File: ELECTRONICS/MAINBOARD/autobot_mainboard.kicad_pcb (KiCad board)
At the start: 4 copper layers, 62 x 42.5 mm, 161 parts, among them IC1 DW3210, J1 USB_C_Receptacle_USB2.0_16P, J10 Conn_01x05_Socket, J12 Conn_01x02_Pin, J14 Conn_01x05_Pin, J16 Conn_01x05_Pin, J17 Conn_01x02_Pin, J18 Conn_01x02_Pin, J19 Conn_02x05_Odd_Even, J20 Conn_02x05_Odd_Even, J7 Conn_01x03_Pin, J8 Conn_Coaxial, J9 Conn_Coaxial, Q1 DMG1012T, Q2 DMG1012T, Q3 DMG1012T, SW1 RESET, SW2 BOOT, U1 TVS1400DRV, U10 VL53L1X, U11 VL53L1X, U12 VL53L1X, U13 BMI270, U14 BMI270, U15 TPD4E05U06DQA, U16 LP5907MFX-3.3, U17 STM32G031C6Tx, U18 LP5907MFX-3.3, U19 STM32H743VITx, U2 LMR51430XDDCR, U22 TPD4E05U06DQA, U23 LP5907MFX-3.3, U3 LP5907MFX-3.3, U4 TPD2EUSB30A, U9 VL53L1X, Y1 TXC 8Y38472012, Y2 25mhz placeholder

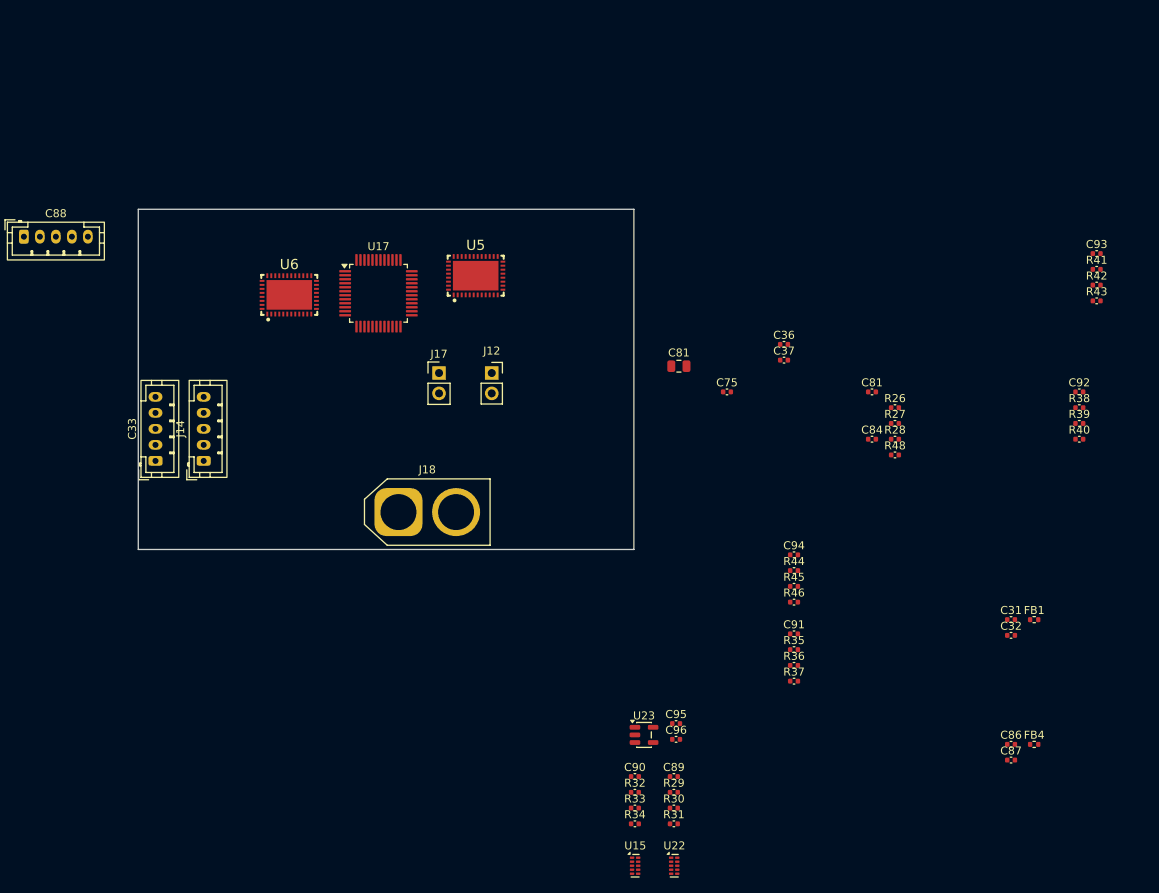
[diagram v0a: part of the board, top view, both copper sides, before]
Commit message: driver board schematic
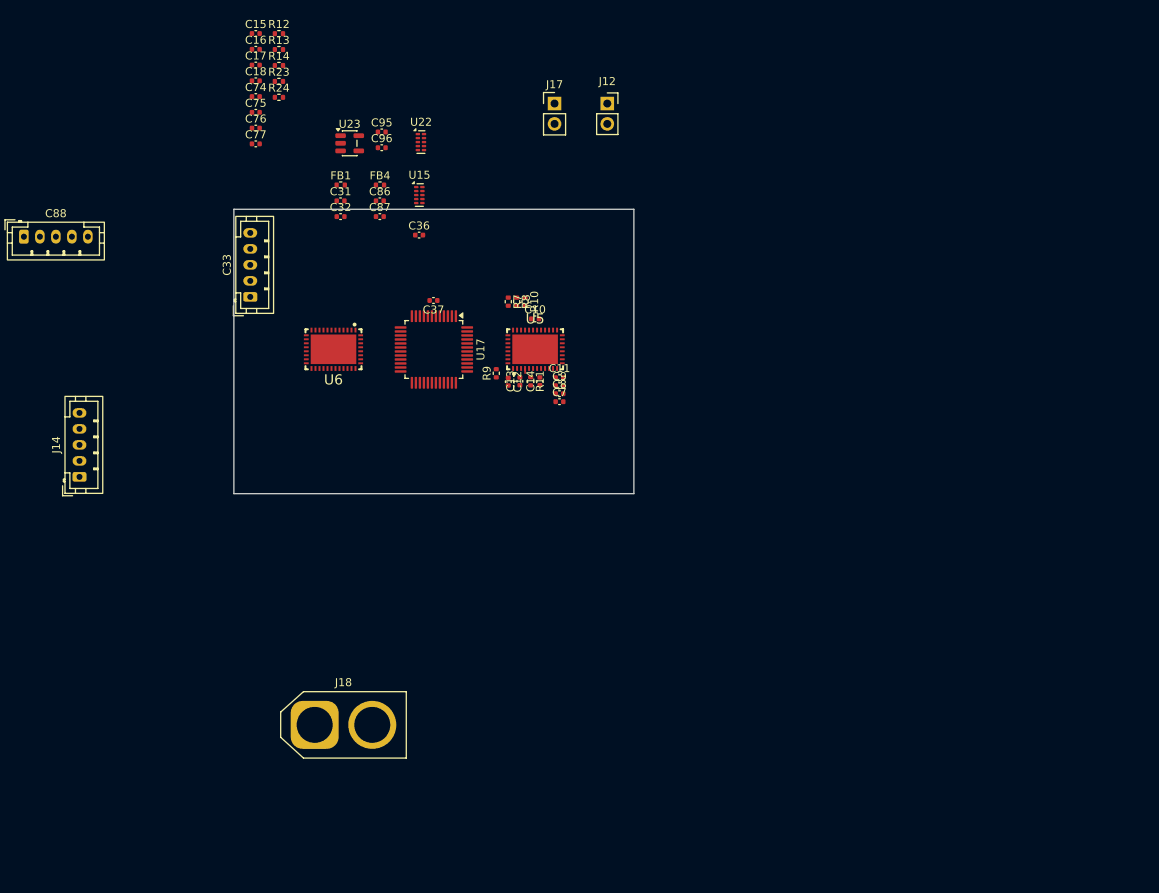
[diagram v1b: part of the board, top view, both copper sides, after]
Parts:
- removed C81: 22u, Capacitor_SMD:C_0402_1005Metric
- removed C81: 22u, Capacitor_SMD:C_0805_2012Metric
- removed C84: 1u, Capacitor_SMD:C_0402_1005Metric
- removed C89, C90, C91, C92, C93, C94: C, Capacitor_SMD:C_0402_1005Metric
- removed R26, R27: 10k, Capacitor_SMD:C_0402_1005Metric
- removed R28, R48: r, Capacitor_SMD:C_0402_1005Metric
- removed R29, R30, R31, R32, R33, R34, R35, R36, R37, R38, R39, R40, R41, R42, R43, R44, R45, R46: 4.7k, Capacitor_SMD:C_0402_1005Metric
- added C10: 1u, Capacitor_SMD:C_0402_1005Metric, F.Cu at (49.6, 33.2)
- added C11: 1u, Capacitor_SMD:C_0402_1005Metric, F.Cu at (52.7, 40.5)
- added C12: 1u, Capacitor_SMD:C_0402_1005Metric, F.Cu at (46.3, 41.0)
- added C13: C, Capacitor_SMD:C_0402_1005Metric, F.Cu at (47.8, 41.0)
- added C14: 47n, Capacitor_SMD:C_0402_1005Metric, F.Cu at (50.2, 41.0)
- added C15: 100u, Capacitor_SMD:C_0402_1005Metric, F.Cu at (14.7, -2.46)
- added C16: 100n, Capacitor_SMD:C_0402_1005Metric, F.Cu at (14.7, -0.49)
- added C17: 100n, Capacitor_SMD:C_0402_1005Metric, F.Cu at (14.7, 1.48)
- added C18: 1u, Capacitor_SMD:C_0402_1005Metric, F.Cu at (14.7, 3.44)
- added C7: 100n, Capacitor_SMD:C_0402_1005Metric, F.Cu at (52.7, 43.5)
- added C74: 1u, Capacitor_SMD:C_0402_1005Metric, F.Cu at (14.7, 5.42)
- added C76: 47n, Capacitor_SMD:C_0402_1005Metric, F.Cu at (14.7, 9.36)
- added C77: C, Capacitor_SMD:C_0402_1005Metric, F.Cu at (14.7, 11.3)
- added C8: 100u, Capacitor_SMD:C_0402_1005Metric, F.Cu at (52.7, 42.5)
- added C9: 100n, Capacitor_SMD:C_0402_1005Metric, F.Cu at (52.7, 41.5)
- added R10: 10K, Resistor_SMD:R_0402_1005Metric, F.Cu at (48.4, 31.1)
- added R11: 22, Resistor_SMD:R_0402_1005Metric, F.Cu at (49.1, 41.0)
- added R12: 10K, Resistor_SMD:R_0402_1005Metric, F.Cu at (17.6, -2.46)
- added R13: 10K, Resistor_SMD:R_0402_1005Metric, F.Cu at (17.6, -0.47)
- added R14: 10K, Resistor_SMD:R_0402_1005Metric, F.Cu at (17.6, 1.52)
- added R23: 10K, Resistor_SMD:R_0402_1005Metric, F.Cu at (17.6, 3.52)
- added R24: 22, Resistor_SMD:R_0402_1005Metric, F.Cu at (17.6, 5.50)
- added R7: 10K, Resistor_SMD:R_0402_1005Metric, F.Cu at (46.3, 31.1)
- added R8: 10K, Resistor_SMD:R_0402_1005Metric, F.Cu at (47.4, 31.1)
- added R9: 10K, Resistor_SMD:R_0402_1005Metric, F.Cu at (44.8, 40.0)
- C75: value 22u -> 1u
- moved FB4 107.6 mm to (30.3, 16.5)
- moved C86 104.1 mm to (30.2, 18.4)
- moved C87 104.1 mm to (30.2, 20.4)
- moved FB1 102.3 mm to (25.4, 16.5)
- moved C31 98.8 mm to (25.3, 18.4)
- moved C32 98.8 mm to (25.3, 20.4)
- moved U22 95.8 mm to (35.4, 11.1)
- moved U15 88.1 mm to (35.2, 17.7)
- moved C95 82.6 mm to (30.5, 9.84)
- moved C96 82.6 mm to (30.5, 11.8)
- moved U23 82.6 mm to (26.5, 11.2)
- moved C75 68.5 mm to (14.7, 7.38)
- moved C36 47.6 mm to (35.2, 22.7)
- moved C37 44.4 mm to (37.0, 30.9), turned to 180 degrees
- moved J12 36.6 mm to (58.7, 6.29)
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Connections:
- C75 pad 1: VDD -> +24V
- C75 pad 2: GNDREF -> Net-(U6-CP)
- U17 pad 11: unconnected-(U17-PA0-Pad11) -> /AMT102_L/AMT_A
- U17 pad 12: unconnected-(U17-PA1-Pad12) -> /AMT102_L/AMT_B
- U17 pad 13: unconnected-(U17-PA2-Pad13) -> /AMT102_L/AMT_X
- U17 pad 16: unconnected-(U17-PA5-Pad16) -> /STM32G0/DACOUT1_R
- U17 pad 17: unconnected-(U17-PA6-Pad17) -> /STM32G0/DACOUT2_R
- U17 pad 18: unconnected-(U17-PA7-Pad18) -> /STM32G0/PWM_R
- U17 pad 19: unconnected-(U17-PB0-Pad19) -> /STM32G0/DIR_R
- U17 pad 20: unconnected-(U17-PB1-Pad20) -> /STM32G0/EXT_WD_R
- U17 pad 21: unconnected-(U17-PB2-Pad21) -> /STM32G0/FG_R
- U17 pad 23: unconnected-(U17-PB11-Pad23) -> /STM32G0/nFAULT_R
- U17 pad 24: unconnected-(U17-PB12-Pad24) -> /STM32G0/DRVOFF_R
- U17 pad 25: unconnected-(U17-PB13-Pad25) -> /STM32G0/BRAKE_R
- U17 pad 28: unconnected-(U17-PA8-Pad28) -> /AMT102_L/AMT_X
- U17 pad 30: unconnected-(U17-PC6-Pad30) -> /AMT102_R/AMT_A
- U17 pad 31: unconnected-(U17-PC7-Pad31) -> /AMT102_R/AMT_B
- U17 pad 38: unconnected-(U17-PD0-Pad38) -> /STM32G0/EXT_WD
- U17 pad 39: unconnected-(U17-PD1-Pad39) -> /STM32G0/BRAKE
- U17 pad 40: unconnected-(U17-PD2-Pad40) -> /STM32G0/DACOUT2
- U17 pad 41: unconnected-(U17-PD3-Pad41) -> /STM32G0/DACOUT1
- U17 pad 42: unconnected-(U17-PB3-Pad42) -> /STM32G0/nFAULT
- U17 pad 43: unconnected-(U17-PB4-Pad43) -> /STM32G0/DRVOFF
- U17 pad 44: unconnected-(U17-PB5-Pad44) -> /STM32G0/DIR
- U17 pad 45: unconnected-(U17-PB6-Pad45) -> /STM32G0/PWM
- U17 pad 46: unconnected-(U17-PB7-Pad46) -> /STM32G0/FG
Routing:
- net VDD: track 11.8 -> 0.00 mm
- net (no net): track 0.00 -> 11.8 mm
- net Net-(U5-GND_BK): track 0.00 -> 0.60 mm
- added copper zone on In2.Cu, net (none)
- removed copper zone on In2.Cu, net VDD
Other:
- board size 62 x 42.5 mm -> 50 x 35.5 mm
